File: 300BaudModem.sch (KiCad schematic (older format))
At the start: 0 parts

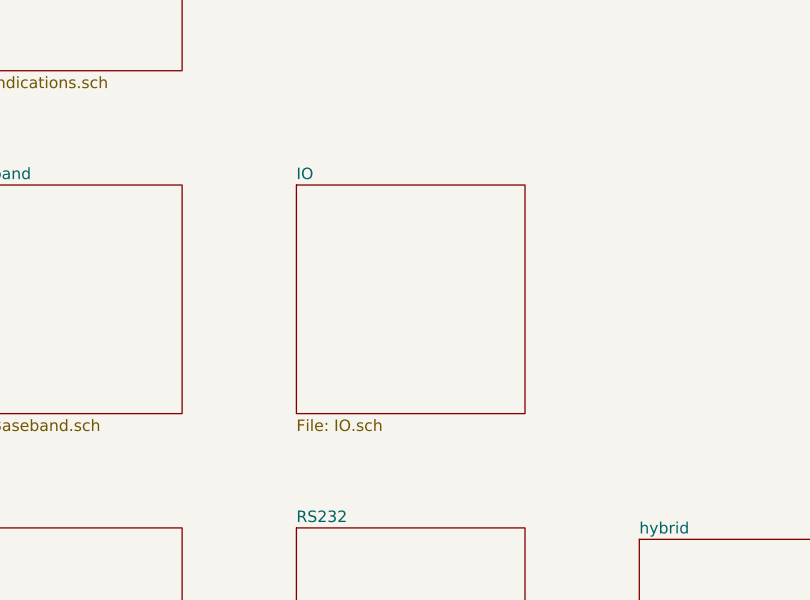
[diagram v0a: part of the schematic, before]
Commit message: updates
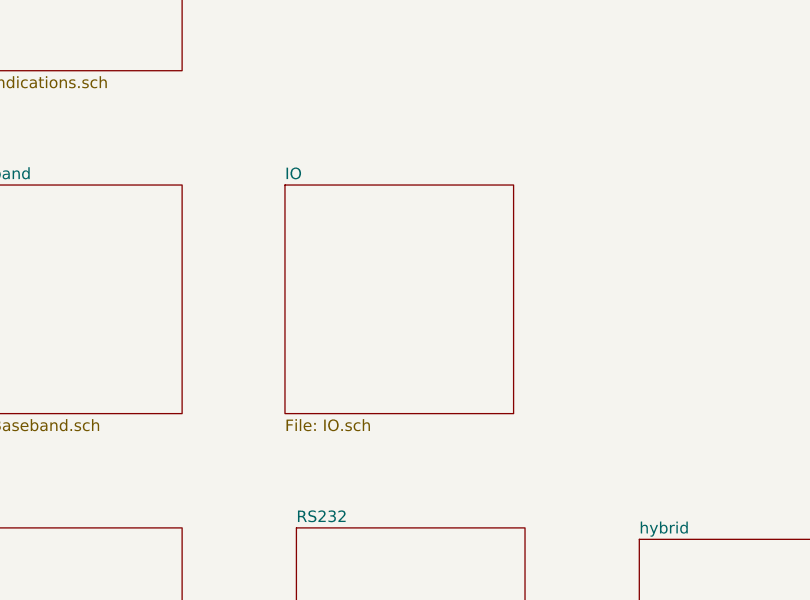
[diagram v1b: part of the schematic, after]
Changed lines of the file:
@@
 $EndSheet
 $Sheet
-S 2500 4000 1000 1000
+S 2450 4000 1000 1000
 U 60E9D9E5
 F0 "IO" 50
